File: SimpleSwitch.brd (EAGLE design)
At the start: 28.9 x 37.5 mm, 36 parts, among them IC3 MC33269ST-3.3T3, K1 FRS1B, T1 BC846, X1 16 MHz

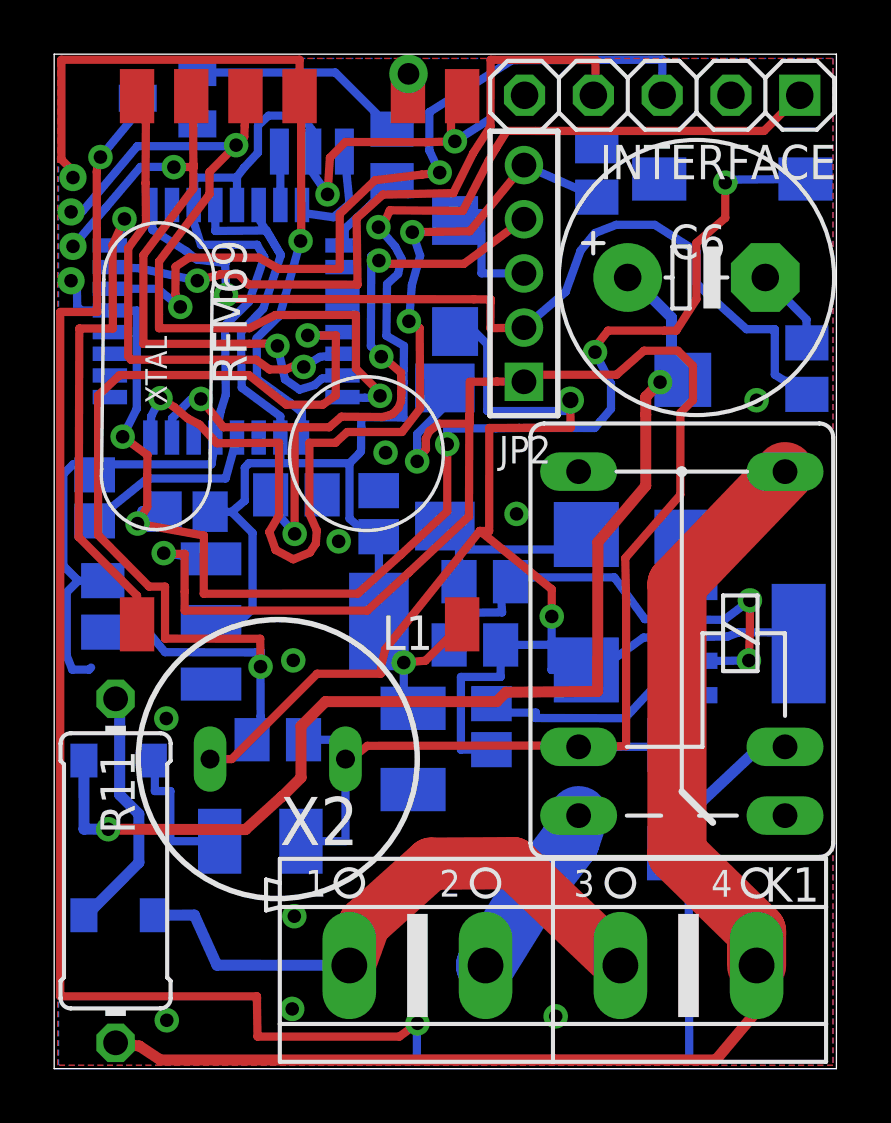
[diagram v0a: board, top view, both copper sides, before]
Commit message: aaa
aaa
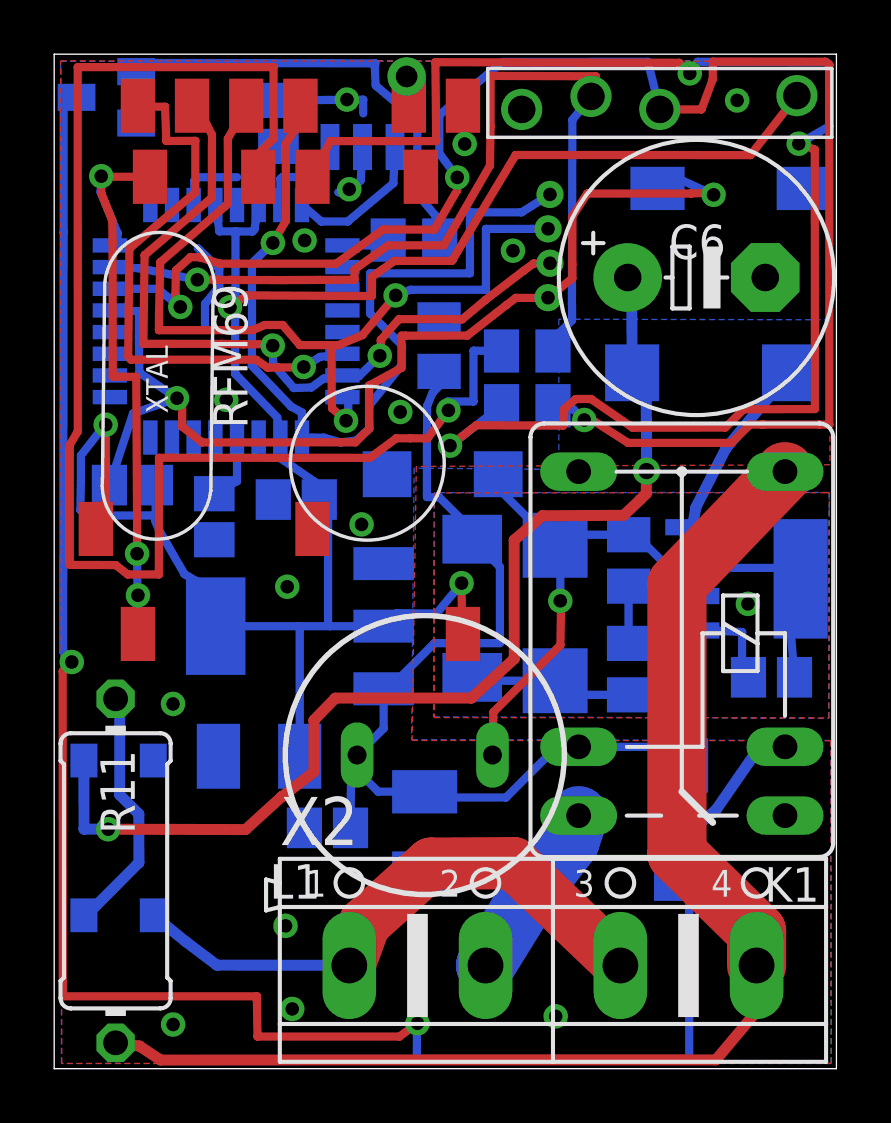
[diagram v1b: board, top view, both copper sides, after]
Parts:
- removed JP2: (no value), pinhead-2:1X05M
- removed R14: 560, resistor:M2012
- removed R3: 10K, resistor:M2012
- removed R5: 20K, resistor:M2012
- added C3, C4: 0.1, resistor:C2012
- added R6: 1 K, resistor:M2012
- added U$5: ESP03, RemoteHome:ESP03
- INTERFACE: value (none) -> PINHD1X5SQUARE; device pinhead-2:1X05-S -> eagle-library-edeca.net-v5:PINHD1X05-SQUARE
- R4: value 470 -> 1K
- R7: value 10K -> 1 K
- RFM69: value RFM69 -> RFM69W; device LowPowerLab:RFM69W-MINPADS -> RemoteHome:RFM69W
- moved U$2 17.6 mm to (18.3, 29.7)
- moved R4 15.7 mm to (14.2, 26.7), turned to 270 degrees
- moved C10 14.9 mm to (8.28, 34.9)
- moved C7 10.5 mm to (26.5, 14.4), turned to 180 degrees
- moved D3 7.33 mm to (14.3, 21.9), turned to 0 degrees
- moved R7 7.11 mm to (17.5, 26.5), turned to 180 degrees
- moved R13 6.48 mm to (21.2, 18.8), turned to 90 degrees
- moved R12 6.21 mm to (21.2, 14.8), turned to 90 degrees
- moved C1 6.08 mm to (13.7, 8.72), turned to 270 degrees
- moved C9 5.69 mm to (7.57, 11.5), turned to 0 degrees
- moved D4 5.68 mm to (15.4, 17.0)
- moved L1 5.43 mm to (13.7, 11.6), turned to 180 degrees
- moved C5 4.47 mm to (5.91, 20.4), turned to 270 degrees
- moved R10 3.32 mm to (24.2, 25.7), turned to 180 degrees
- moved R2 3.25 mm to (13.3, 30.6), turned to 180 degrees
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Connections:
- net N$10 renamed S
- new net N$10: R6.1, U$5.WIFI_TX
- new net N$11: R7.1, U$5.WIFI_RX
- net 5V: now also C3.1; no longer JP2.1
- net A0: no longer JP2.4, R5.2
- net A1: no longer JP2.5, R7.2
- net D0_RX: now also R6.2
- net D1_TX: now also R7.2
- net D2: now also U$5.WIFI_EN
- net D3: no longer JP2.2, R3.2
- net D9: no longer R14.2, R4.1
- net GND: now also C3.2, C4.2, R4.1, U$5.WIFI_GND, U$5.WIFI_GPIO15; no longer JP2.3, R14.1, R3.1, R5.1, R7.1
- net VCC: now also C4.1, U$5.WIFI_VDD
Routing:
- net N$10: track 0.00 -> 54.5 mm, vias 0 -> 3
- net N$11: track 0.00 -> 53.3 mm, vias 0 -> 1
- net GND: track 64.6 -> 13.3 mm, vias 12 -> 15
- net D9: track 39.3 -> 0.00 mm, vias 2 -> 0
- net A1: track 35.9 -> 0.00 mm, vias 3 -> 0
- net 5V: track 73.3 -> 37.7 mm, vias 2 -> 0
- net D3: track 33.7 -> 0.00 mm, vias 1 -> 0
- net D0_RX: track 29.6 -> 61.2 mm, vias 2 -> 3
- net A0: track 28.7 -> 0.00 mm, vias 4 -> 0
- net S: track 56.5 -> 27.9 mm
- net FB: track 19.4 -> 4.60 mm, vias 2 -> 0
- net RST: track 52.6 -> 39.4 mm, vias 5 -> 2
- net VCC: track 70.5 -> 80.3 mm, vias 2 -> 3
- net N$2: track 8.05 -> 17.3 mm
- net D1_TX: track 26.2 -> 34.4 mm
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- added copper zone on layer 1, net S
- added copper zone on layer 16, net S
